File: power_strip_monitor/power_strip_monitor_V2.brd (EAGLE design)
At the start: 100 x 80 mm, 72 parts, among them IC2 ATMEGA644A, J1 EXP, Q1 16.384MHz, Q2 BTA312B-800E, Q3 BTA312B-800E, Q4 BTA312B-800E, Q5 BTA312B-800E, Q6 BTA312B-800E, Q7 BTA312B-800E, U1 CS5467, U10 LTP5901, U2 CS5467, U3 CS5467, U5 RAC01_02-SC, U8 SN74VC4245A, U9 SN74VC4245A

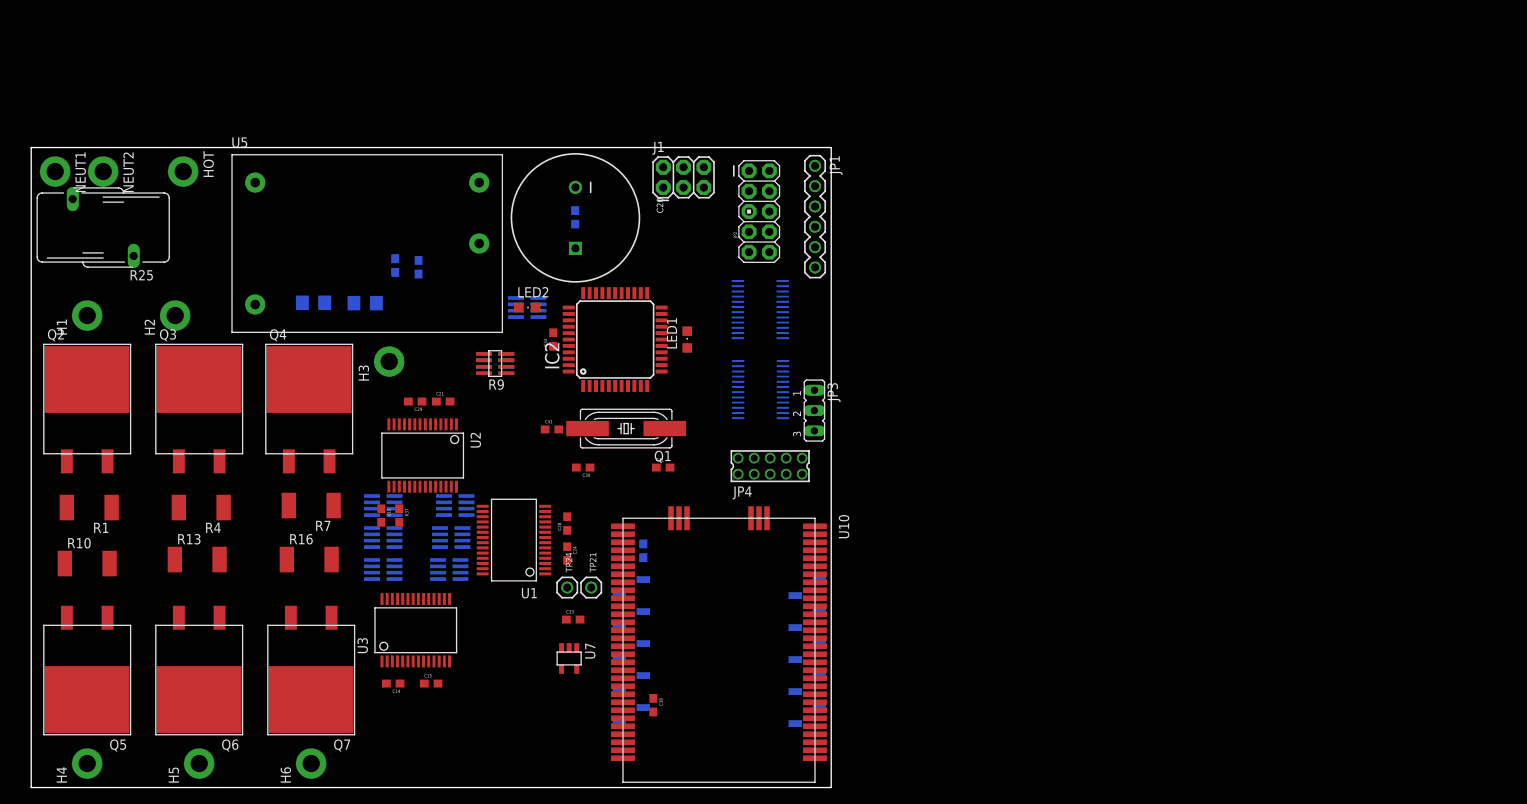
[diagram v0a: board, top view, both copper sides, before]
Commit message: Ready to route
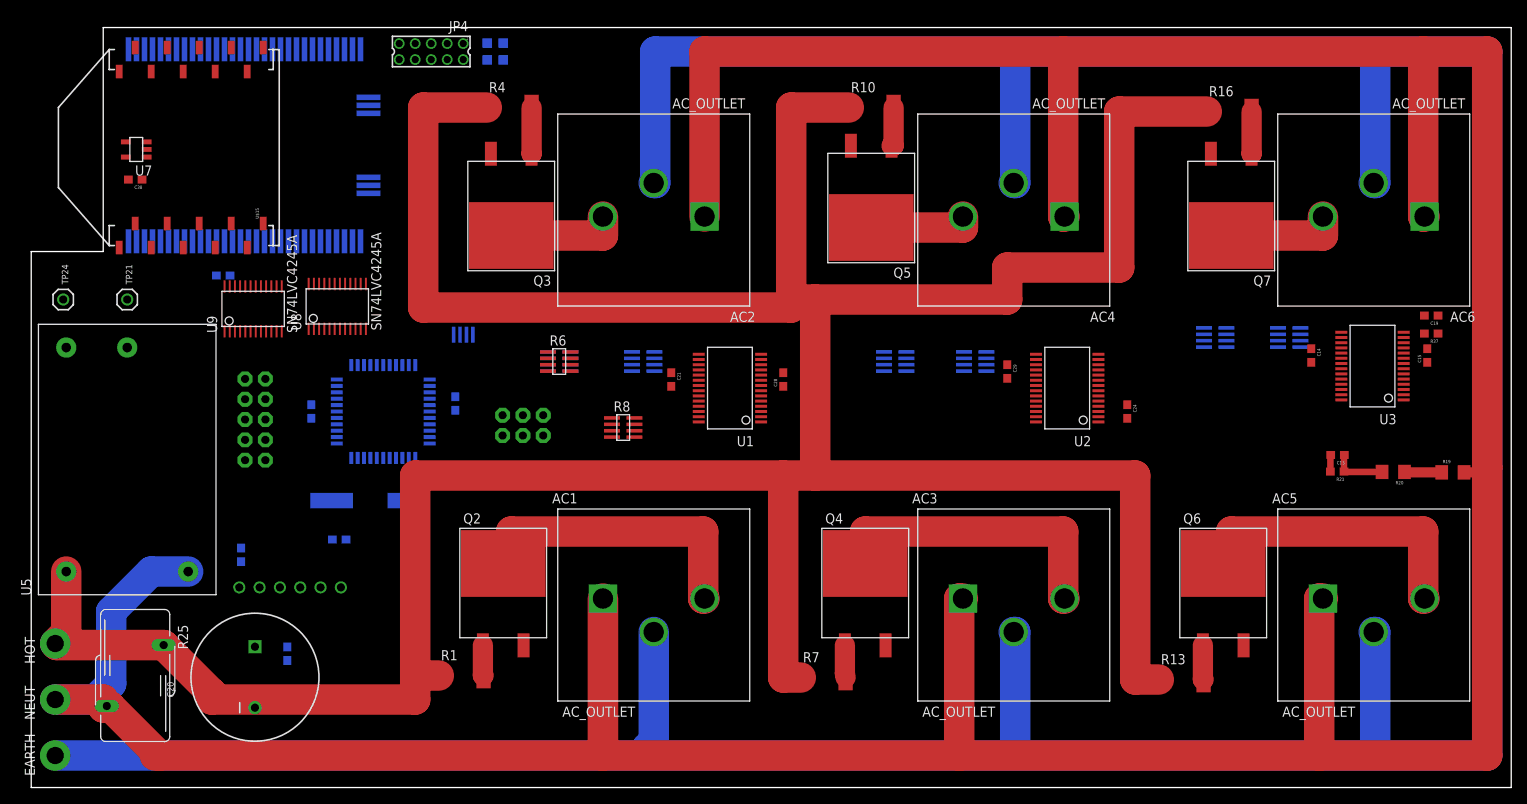
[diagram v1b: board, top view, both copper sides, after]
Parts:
- removed H1, H2, H3, H4, H5, H6, NEUT1, NEUT2: 1P_HOLE, Cool_Electricity:14GAUGE_HOLE
- removed JP3: (no value), jumper:JP2
- added AC1, AC2, AC3, AC4, AC5, AC6: AC_OUTLET, Cool_Electricity:3-213598-2
- added EARTH, NEUT: 1P_HOLE, Cool_Electricity:14GAUGE_HOLE
- U8, U9: value SN74VC4245A -> SN74LVC4245A
- moved R19 144.0 mm to (177.7, 39.4), flipped to the top
- moved C19 133.6 mm to (175.0, 59.0), turned to 180 degrees
- moved C15 131.1 mm to (174.5, 54.0), turned to 90 degrees
- moved R37 131.0 mm to (175.0, 56.8), turned to 180 degrees
- moved R20 130.2 mm to (170.3, 39.5), flipped to the top
- moved Q6 129.1 mm to (149.0, 28.0), turned to 0 degrees
- moved Q7 128.8 mm to (150.0, 69.0)
- moved R16 127.9 mm to (149.8, 84.5)
- moved U3 124.1 mm to (167.7, 52.7), turned to 180 degrees
- moved R13 123.9 mm to (143.8, 13.5)
- moved C14 121.9 mm to (160.0, 54.0), turned to 270 degrees
- moved R21 120.5 mm to (163.2, 39.5), flipped to the top, turned to 180 degrees
- moved C13 117.2 mm to (163.3, 41.6), flipped to the top, turned to 180 degrees
- moved Q5 114.4 mm to (105.0, 70.0)
- moved R10 113.4 mm to (105.0, 85.0)
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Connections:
- removed net N$18: H2.P$1, Q3.2
- removed net N$20: H3.P$1, Q4.2
- removed net N$21: H4.P$1, Q5.2
- removed net N$23: H5.P$1, Q6.2
- removed net N$25: H6.P$1, Q7.2
- removed net N$5: JP3.2, U8.22, U9.22
- removed net N$9: H1.P$1, Q2.2
- new net EARTH: AC1.3, AC2.3, AC3.3, AC4.3, AC5.3, AC6.3, EARTH.P$1
- new net HOT1: AC1.2, Q2.2
- new net HOT2: AC2.2, Q3.2
- new net HOT3: AC3.2, Q4.2
- new net HOT4: AC4.2, Q5.2
- new net HOT5: AC5.2, Q6.2
- new net HOT6: AC6.2, Q7.2
- net 5V: now also U8.22; no longer JP3.3
- net GND: now also U9.22; no longer JP3.1
- net NEUTRAL: now also AC1.1, AC2.1, AC3.1, AC4.1, AC5.1, AC6.1, NEUT.P$1; no longer NEUT1.P$1, NEUT2.P$1
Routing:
- net NEUTRAL: track 0.00 -> 522.8 mm
- net EARTH: track 0.00 -> 470.2 mm
- net GND: track 0.00 -> 445.5 mm
- net HOT1: track 0.00 -> 39.5 mm
- net HOT5: track 0.00 -> 37.5 mm
- net HOT3: track 0.00 -> 37.3 mm
- net HOT2: track 0.00 -> 13.8 mm
- net HOT6: track 0.00 -> 13.8 mm
- net HOT4: track 0.00 -> 12.8 mm
- net V+: track 0.00 -> 6.85 mm
- net HRET2: track 0.00 -> 5.79 mm
- net HRET6: track 0.00 -> 5.29 mm
- net HRET4: track 0.00 -> 5.03 mm
- net N$2: track 0.00 -> 4.67 mm
- net HRET5: track 0.00 -> 4.37 mm
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- removed copper zone on layer 15, net 5V
- removed copper zone on layer 2, net GND
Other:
- board size 100 x 80 mm -> 185 x 95 mm
- board text added: "SOLDER 14AWG WIRE ON BUS"
